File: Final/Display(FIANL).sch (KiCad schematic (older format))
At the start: 25 parts, among them U31 PAL16L8, U32 PAL16L8, U33 74LS374, U34 74LS374, U35 74LS374, U36 MAN71A, U37 MAN71A

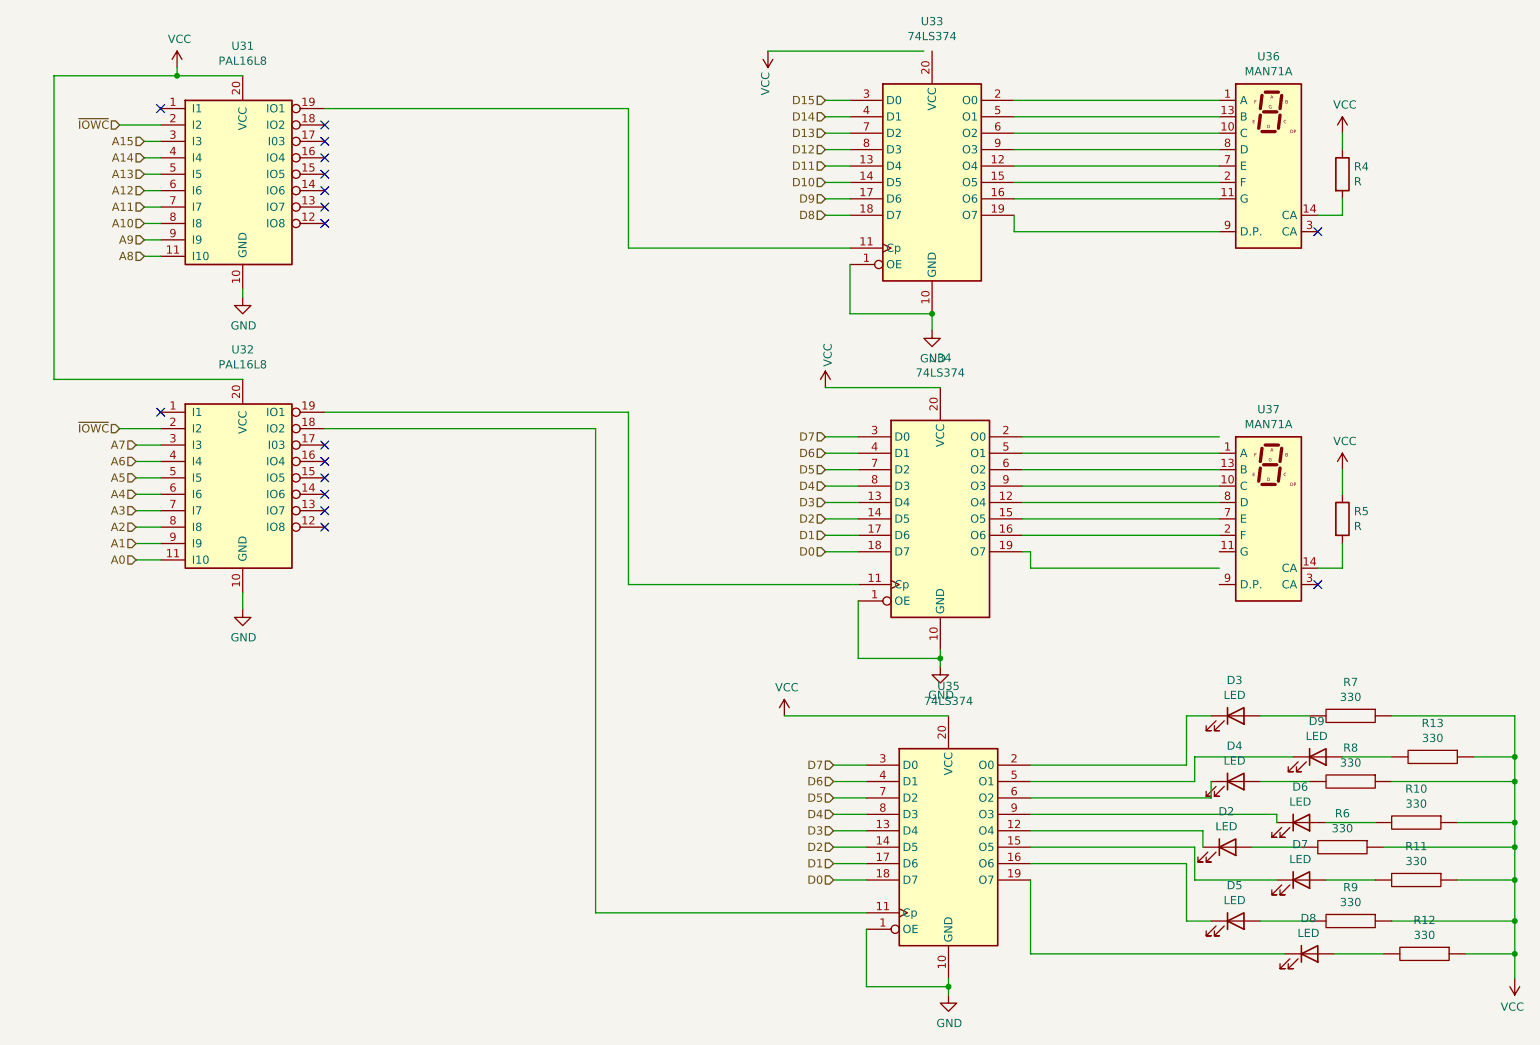
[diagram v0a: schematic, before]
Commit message: Final?
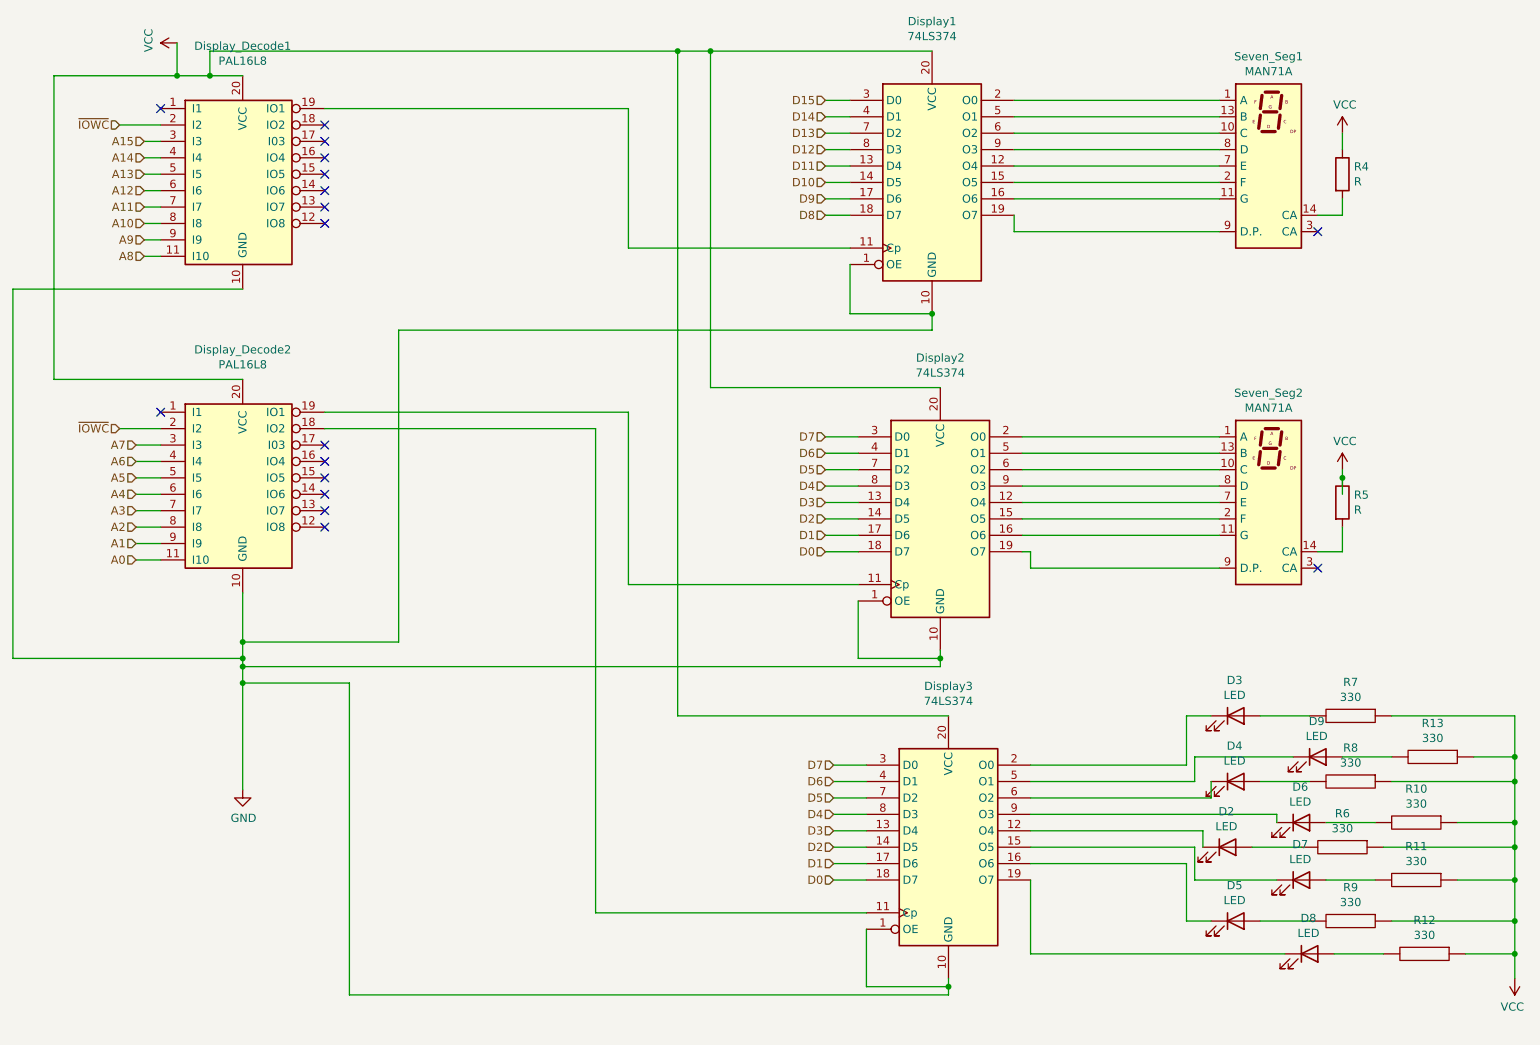
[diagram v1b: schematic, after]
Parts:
- renumbered U33 to Display1, U34 to Display2, U35 to Display3, U31 to Display_Decode1, U32 to Display_Decode2, U36 to Seven_Seg1, U37 to Seven_Seg2
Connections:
- net VCC: now also Display1.20 (VCC)
- net at Display2.12 (O4): now also Seven_Seg2.7 (E); no longer Seven_Seg2.8 (D)
- net at Display2.15 (O5): now also Seven_Seg2.2 (F); no longer Seven_Seg2.7 (E)
- net at Display2.16 (O6): now also Seven_Seg2.11 (G); no longer Seven_Seg2.2 (F)
- net at Display2.19 (O7): now also Seven_Seg2.9 (D.P.)
- net at Display2.2 (O0): now also Seven_Seg2.1 (A)
- net at Display2.5 (O1): now also Seven_Seg2.13 (B); no longer Seven_Seg2.1 (A)
- net at Display2.6 (O2): now also Seven_Seg2.10 (C); no longer Seven_Seg2.13 (B)
- net at Display2.9 (O3): now also Seven_Seg2.8 (D); no longer Seven_Seg2.10 (C)
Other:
- moved on the sheet: R5, Seven_Seg2
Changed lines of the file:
@@
 $Descr A4 11693 8268
 encoding utf-8
-Sheet 11 16
+Sheet 13 16
 Title ""
 Date ""
@@
 $EndDescr
 $Comp
-L 74xx:74LS374 U33
+L 74xx:74LS374 Display1
 U 1 1 607791B4
 P 7500 1450
-F 0 "U33" H 7500 2431 50  0000 C CNN
+F 0 "Display1" H 7500 2431 50  0000 C CNN
 F 1 "74LS374" H 7500 2340 50  0000 C CNN
 F 2 "" H 7500 1450 50  0001 C CNN
@@
 $EndComp
 $Comp
-L 74xx:74LS374 U34
+L 74xx:74LS374 Display2
 U 1 1 60775947
 P 7550 3500
-F 0 "U34" H 7550 4481 50  0000 C CNN
+F 0 "Display2" H 7550 4481 50  0000 C CNN
 F 1 "74LS374" H 7550 4390 50  0000 C CNN
 F 2 "" H 7550 3500 50  0001 C CNN
@@
 $EndComp
 $Comp
-L 74xx:74LS374 U35
+L 74xx:74LS374 Display3
 U 1 1 60778C07
 P 7600 5500
-F 0 "U35" H 7600 6481 50  0000 C CNN
+F 0 "Display3" H 7600 6481 50  0000 C CNN
 F 1 "74LS374" H 7600 6390 50  0000 C CNN
 F 2 "" H 7600 5500 50  0001 C CNN
@@
 Wire Wire Line
 	7100 5100 6900 5100
-$Comp
-L power:VCC #PWR057
-U 1 1 6079D8CA
-P 6850 2700
-F 0 "#PWR057" H 6850 2550 50  0001 C CNN
-F 1 "VCC" V 6865 2827 50  0000 L CNN
-F 2 "" H 6850 2700 50  0001 C CNN
-F 3 "" H 6850 2700 50  0001 C CNN
-	1    6850 2700
-	1    0    0    -1
-$EndComp
-$Comp
-L power:GND #PWR058
-U 1 1 607A1D53
-P 7600 6400
-F 0 "#PWR058" H 7600 6150 50  0001 C CNN
-F 1 "GND" H 7605 6227 50  0000 C CNN
-F 2 "" H 7600 6400 50  0001 C CNN
-F 3 "" H 7600 6400 50  0001 C CNN
-	1    7600 6400
-	1    0    0    -1
-$EndComp
 Wire Wire Line
 	7000 1950 7000 2250
@@
 	7050 4350 7550 4350
 $Comp
-L Display_Character:MAN71A U36
+L Display_Character:MAN71A Seven_Seg1
 U 1 1 6078B9DF
 P 9550 1350
-F 0 "U36" H 9550 2017 50  0000 C CNN
+F 0 "Seven_Seg1" H 9550 2017 50  0000 C CNN
 F 1 "MAN71A" H 9550 1926 50  0000 C CNN
 F 2 "Display_7Segment:MAN71A" H 9050 650 50  0001 L CNN
@@
 $EndComp
 $Comp
-L Display_Character:MAN71A U37
+L Display_Character:MAN71A Seven_Seg2
 U 1 1 6079109D
-P 9550 3500
-F 0 "U37" H 9550 4167 50  0000 C CNN
-F 1 "MAN71A" H 9550 4076 50  0000 C CNN
-F 2 "Display_7Segment:MAN71A" H 9050 2800 50  0001 L CNN
-F 3 "https://www.digchip.com/datasheets/parts/datasheet/161/MAN3640A-pdf.php" H 9560 3840 50  0001 L CNN
-	1    9550 3500
+P 9550 3400
+F 0 "Seven_Seg2" H 9550 4067 50  0000 C CNN
+F 1 "MAN71A" H 9550 3976 50  0000 C CNN
+F 2 "Display_7Segment:MAN71A" H 9050 2700 50  0001 L CNN
+F 3 "https://www.digchip.com/datasheets/parts/datasheet/161/MAN3640A-pdf.php" H 9560 3740 50  0001 L CNN
+	1    9550 3400
 	1    0    0    -1
 $EndComp
@@
 	5650 1850 7000 1850
 Wire Wire Line
-	3300 800  2900 800
-Wire Wire Line
-	2900 800  2900 750
+	3300 800  3100 800
 $Comp
 L power:VCC #PWR054
 U 1 1 607ECC89
-P 2900 750
-F 0 "#PWR054" H 2900 600 50  0001 C CNN
-F 1 "VCC" H 2915 923 50  0000 C CNN
-F 2 "" H 2900 750 50  0001 C CNN
-F 3 "" H 2900 750 50  0001 C CNN
-	1    2900 750
-	1    0    0    -1
-$EndComp
-$Comp
-L power:GND #PWR055
-U 1 1 607EDAEB
-P 3300 2150
-F 0 "#PWR055" H 3300 1900 50  0001 C CNN
-F 1 "GND" H 3305 1977 50  0000 C CNN
-F 2 "" H 3300 2150 50  0001 C CNN
-F 3 "" H 3300 2150 50  0001 C CNN
-	1    3300 2150
-	1    0    0    -1
+P 2900 600
+F 0 "#PWR054" H 2900 450 50  0001 C CNN
+F 1 "VCC" H 2915 773 50  0000 C CNN
+F 2 "" H 2900 600 50  0001 C CNN
+F 3 "" H 2900 600 50  0001 C CNN
+	1    2900 600
+	0    -1   -1   0
 $EndComp
 Wire Wire Line
 	2800 1100 2550 1100
 $Comp
-L Logic_Programmable:PAL16L8 U32
+L Logic_Programmable:PAL16L8 Display_Decode2
 U 1 1 607F2271
 P 3300 3350
-F 0 "U32" H 3300 4231 50  0000 C CNN
+F 0 "Display_Decode2" H 3300 4231 50  0000 C CNN
 F 1 "PAL16L8" H 3300 4140 50  0000 C CNN
 F 2 "" H 3300 3350 50  0001 C CNN
@@
 	2150 800  2900 800
 Connection ~ 2900 800
-Wire Wire Line
-	3300 2100 3300 2150
-Wire Wire Line
-	3300 3950 3300 4050
 $Comp
 L power:GND #PWR056
 U 1 1 607FE1E1
-P 3300 4050
-F 0 "#PWR056" H 3300 3800 50  0001 C CNN
-F 1 "GND" H 3305 3877 50  0000 C CNN
-F 2 "" H 3300 4050 50  0001 C CNN
-F 3 "" H 3300 4050 50  0001 C CNN
-	1    3300 4050
+P 3300 5150
+F 0 "#PWR056" H 3300 4900 50  0001 C CNN
+F 1 "GND" H 3305 4977 50  0000 C CNN
+F 2 "" H 3300 5150 50  0001 C CNN
+F 3 "" H 3300 5150 50  0001 C CNN
+	1    3300 5150
 	1    0    0    -1
 $EndComp
@@
 	2800 2950 2550 2950
 $Comp
-L Logic_Programmable:PAL16L8 U31
+L Logic_Programmable:PAL16L8 Display_Decode1
 U 1 1 607E2663
 P 3300 1500
-F 0 "U31" H 3300 2381 50  0000 C CNN
+F 0 "Display_Decode1" H 3300 2381 50  0000 C CNN
 F 1 "PAL16L8" H 3300 2290 50  0000 C CNN
 F 2 "" H 3300 1500 50  0001 C CNN
@@
 	10000 1650 10000 1550
 Wire Wire Line
-	9850 3800 10000 3800
-Wire Wire Line
-	10000 3800 10000 3650
+	9850 3700 10000 3700
+Wire Wire Line
+	10000 3700 10000 3550
 $Comp
 L Device:R R4
@@
 L Device:R R5
 U 1 1 607D65C2
-P 10000 3500
-F 0 "R5" H 10070 3546 50  0000 L CNN
-F 1 "R" H 10070 3455 50  0000 L CNN
-F 2 "" V 9930 3500 50  0001 C CNN
-F 3 "~" H 10000 3500 50  0001 C CNN
-	1    10000 3500
+P 10000 3400
+F 0 "R5" H 10070 3446 50  0000 L CNN
+F 1 "R" H 10070 3355 50  0000 L CNN
+F 2 "" V 9930 3400 50  0001 C CNN
+F 3 "~" H 10000 3400 50  0001 C CNN
+	1    10000 3400
 	1    0    0    -1
 $EndComp
@@
 	10000 1250 10000 1150
 Wire Wire Line
-	10000 3350 10000 3200
+	10000 3350 10000 3250
 $Comp
 L power:VCC #PWR059
@@
 NoConn ~ 3800 3550
 NoConn ~ 9850 1750
-NoConn ~ 9850 3900
 Wire Wire Line
 	5450 2950 5450 5900
@@
 	7550 4350 7550 4300
 Connection ~ 7550 4350
-$Comp
-L power:GND #PWR0105
-U 1 1 60A72376
-P 7550 4400
-F 0 "#PWR0105" H 7550 4150 50  0001 C CNN
-F 1 "GND" H 7555 4227 50  0000 C CNN
-F 2 "" H 7550 4400 50  0001 C CNN
-F 3 "" H 7550 4400 50  0001 C CNN
-	1    7550 4400
-	1    0    0    -1
-$EndComp
-$Comp
-L power:GND #PWR0102
-U 1 1 60A729AF
-P 7500 2350
-F 0 "#PWR0102" H 7500 2100 50  0001 C CNN
-F 1 "GND" H 7505 2177 50  0000 C CNN
-F 2 "" H 7500 2350 50  0001 C CNN
-F 3 "" H 7500 2350 50  0001 C CNN
-	1    7500 2350
-	1    0    0    -1
-$EndComp
-Wire Wire Line
-	7450 650  6500 650
-Wire Wire Line
-	7550 2700 6850 2700
-Wire Wire Line
-	7600 4700 6600 4700
-$Comp
-L power:VCC #PWR0103
-U 1 1 60A94EE1
-P 6600 4700
-F 0 "#PWR0103" H 6600 4550 50  0001 C CNN
-F 1 "VCC" H 6615 4873 50  0000 C CNN
-F 2 "" H 6600 4700 50  0001 C CNN
-F 3 "" H 6600 4700 50  0001 C CNN
-	1    6600 4700
-	1    0    0    -1
-$EndComp
-$Comp
-L power:VCC #PWR0104
-U 1 1 60A9BDC3
-P 6500 650
-F 0 "#PWR0104" H 6500 500 50  0001 C CNN
-F 1 "VCC" V 6515 777 50  0000 L CNN
-F 2 "" H 6500 650 50  0001 C CNN
-F 3 "" H 6500 650 50  0001 C CNN
-	1    6500 650
-	-1   0    0    1
-$EndComp
+Wire Wire Line
+	3300 3950 3300 4250
+Wire Wire Line
+	3300 2100 1900 2100
+Wire Wire Line
+	1900 2100 1900 4350
+Wire Wire Line
+	1900 4350 3300 4350
+Connection ~ 3300 4350
+Wire Wire Line
+	3300 4350 3300 4400
+Wire Wire Line
+	2900 600  2900 800
+Wire Wire Line
+	3100 650  3100 800
+Connection ~ 3100 800
+Wire Wire Line
+	3100 800  2900 800
+Wire Wire Line
+	3100 650  5950 650
+Wire Wire Line
+	7600 6400 3950 6400
+Wire Wire Line
+	3950 6400 3950 4500
+Wire Wire Line
+	3950 4500 3300 4500
+Connection ~ 3300 4500
+Wire Wire Line
+	7550 4400 3300 4400
+Connection ~ 3300 4400
+Wire Wire Line
+	3300 4400 3300 4500
+Wire Wire Line
+	7500 2350 4250 2350
+Wire Wire Line
+	4250 2350 4250 4250
+Wire Wire Line
+	4250 4250 3300 4250
+Connection ~ 3300 4250
+Wire Wire Line
+	3300 4250 3300 4350
+Wire Wire Line
+	3300 4500 3300 5150
+Wire Wire Line
+	6150 2700 6150 650
+Wire Wire Line
+	6150 2700 7550 2700
+Connection ~ 6150 650
+Wire Wire Line
+	6150 650  7500 650
+Wire Wire Line
+	5950 4700 5950 650
+Wire Wire Line
+	5950 4700 7600 4700
+Connection ~ 5950 650
+Wire Wire Line
+	5950 650  6150 650
+Connection ~ 10000 3250
+Wire Wire Line
+	10000 3250 10000 3200
+NoConn ~ 9850 3800
 $EndSCHEMATC

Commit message: Hopefully the board is here
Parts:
- D2, D3, D4, D5, D6, D7, D8, D9: footprint (none) -> LED_THT:LED_D1.8mm_W1.8mm_H2.4mm_Horizontal_O1.27mm_Z4.9mm
- Display1, Display2, Display3, Display_Decode1, Display_Decode2: footprint (none) -> Package_DIP:DIP-20_W7.62mm
- R10, R11, R12, R13, R4, R5, R6, R7, R8, R9: footprint (none) -> Resistor_THT:R_Axial_DIN0204_L3.6mm_D1.6mm_P2.54mm_Vertical
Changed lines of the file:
@@
 F 0 "Display1" H 7500 2431 50  0000 C CNN
 F 1 "74LS374" H 7500 2340 50  0000 C CNN
-F 2 "" H 7500 1450 50  0001 C CNN
+F 2 "Package_DIP:DIP-20_W7.62mm" H 7500 1450 50  0001 C CNN
 F 3 "http://www.ti.com/lit/gpn/sn74LS374" H 7500 1450 50  0001 C CNN
 	1    7500 1450
@@
 F 0 "Display2" H 7550 4481 50  0000 C CNN
 F 1 "74LS374" H 7550 4390 50  0000 C CNN
-F 2 "" H 7550 3500 50  0001 C CNN
+F 2 "Package_DIP:DIP-20_W7.62mm" H 7550 3500 50  0001 C CNN
 F 3 "http://www.ti.com/lit/gpn/sn74LS374" H 7550 3500 50  0001 C CNN
 	1    7550 3500
@@
 F 0 "Display3" H 7600 6481 50  0000 C CNN
 F 1 "74LS374" H 7600 6390 50  0000 C CNN
-F 2 "" H 7600 5500 50  0001 C CNN
+F 2 "Package_DIP:DIP-20_W7.62mm" H 7600 5500 50  0001 C CNN
 F 3 "http://www.ti.com/lit/gpn/sn74LS374" H 7600 5500 50  0001 C CNN
 	1    7600 5500
@@
 F 0 "Display_Decode2" H 3300 4231 50  0000 C CNN
 F 1 "PAL16L8" H 3300 4140 50  0000 C CNN
-F 2 "" H 3300 3350 50  0001 C CNN
+F 2 "Package_DIP:DIP-20_W7.62mm" H 3300 3350 50  0001 C CNN
 F 3 "" H 3300 3350 50  0001 C CNN
 	1    3300 3350
@@
 F 0 "Display_Decode1" H 3300 2381 50  0000 C CNN
 F 1 "PAL16L8" H 3300 2290 50  0000 C CNN
-F 2 "" H 3300 1500 50  0001 C CNN
+F 2 "Package_DIP:DIP-20_W7.62mm" H 3300 1500 50  0001 C CNN
 F 3 "" H 3300 1500 50  0001 C CNN
 	1    3300 1500
@@
 F 0 "R7" V 9845 4700 50  0000 C CNN
 F 1 "330" V 9936 4700 50  0000 C CNN
-F 2 "" H 10050 4700 50  0001 C CNN
+F 2 "Resistor_THT:R_Axial_DIN0204_L3.6mm_D1.6mm_P2.54mm_Vertical" H 10050 4700 50  0001 C CNN
 F 3 "~" H 10050 4700 50  0001 C CNN
 	1    10050 4700
@@
 F 0 "R13" V 10345 4950 50  0000 C CNN
 F 1 "330" V 10436 4950 50  0000 C CNN
-F 2 "" H 10550 4950 50  0001 C CNN
+F 2 "Resistor_THT:R_Axial_DIN0204_L3.6mm_D1.6mm_P2.54mm_Vertical" H 10550 4950 50  0001 C CNN
 F 3 "~" H 10550 4950 50  0001 C CNN
 	1    10550 4950
@@
 F 0 "R8" V 9845 5100 50  0000 C CNN
 F 1 "330" V 9936 5100 50  0000 C CNN
-F 2 "" H 10050 5100 50  0001 C CNN
+F 2 "Resistor_THT:R_Axial_DIN0204_L3.6mm_D1.6mm_P2.54mm_Vertical" H 10050 5100 50  0001 C CNN
 F 3 "~" H 10050 5100 50  0001 C CNN
 	1    10050 5100
@@
 F 0 "R10" V 10245 5350 50  0000 C CNN
 F 1 "330" V 10336 5350 50  0000 C CNN
-F 2 "" H 10450 5350 50  0001 C CNN
+F 2 "Resistor_THT:R_Axial_DIN0204_L3.6mm_D1.6mm_P2.54mm_Vertical" H 10450 5350 50  0001 C CNN
 F 3 "~" H 10450 5350 50  0001 C CNN
 	1    10450 5350
@@
 F 0 "R11" V 10245 5700 50  0000 C CNN
 F 1 "330" V 10336 5700 50  0000 C CNN
-F 2 "" H 10450 5700 50  0001 C CNN
+F 2 "Resistor_THT:R_Axial_DIN0204_L3.6mm_D1.6mm_P2.54mm_Vertical" H 10450 5700 50  0001 C CNN
 F 3 "~" H 10450 5700 50  0001 C CNN
 	1    10450 5700
@@
 F 0 "R6" V 9795 5500 50  0000 C CNN
 F 1 "330" V 9886 5500 50  0000 C CNN
-F 2 "" H 10000 5500 50  0001 C CNN
+F 2 "Resistor_THT:R_Axial_DIN0204_L3.6mm_D1.6mm_P2.54mm_Vertical" H 10000 5500 50  0001 C CNN
 F 3 "~" H 10000 5500 50  0001 C CNN
 	1    10000 5500
@@
 F 0 "R9" V 9845 5950 50  0000 C CNN
 F 1 "330" V 9936 5950 50  0000 C CNN
-F 2 "" H 10050 5950 50  0001 C CNN
+F 2 "Resistor_THT:R_Axial_DIN0204_L3.6mm_D1.6mm_P2.54mm_Vertical" H 10050 5950 50  0001 C CNN
 F 3 "~" H 10050 5950 50  0001 C CNN
 	1    10050 5950
@@
 F 0 "R12" V 10295 6150 50  0000 C CNN
 F 1 "330" V 10386 6150 50  0000 C CNN
-F 2 "" H 10500 6150 50  0001 C CNN
+F 2 "Resistor_THT:R_Axial_DIN0204_L3.6mm_D1.6mm_P2.54mm_Vertical" H 10500 6150 50  0001 C CNN
 F 3 "~" H 10500 6150 50  0001 C CNN
 	1    10500 6150
@@
 F 0 "D3" H 9343 4917 50  0000 C CNN
 F 1 "LED" H 9343 4826 50  0000 C CNN
-F 2 "" H 9350 4700 50  0001 C CNN
+F 2 "LED_THT:LED_D1.8mm_W1.8mm_H2.4mm_Horizontal_O1.27mm_Z4.9mm" H 9350 4700 50  0001 C CNN
 F 3 "~" H 9350 4700 50  0001 C CNN
 	1    9350 4700
@@
 F 0 "D5" H 9343 6167 50  0000 C CNN
 F 1 "LED" H 9343 6076 50  0000 C CNN
-F 2 "" H 9350 5950 50  0001 C CNN
+F 2 "LED_THT:LED_D1.8mm_W1.8mm_H2.4mm_Horizontal_O1.27mm_Z4.9mm" H 9350 5950 50  0001 C CNN
 F 3 "~" H 9350 5950 50  0001 C CNN
 	1    9350 5950
@@
 F 0 "D4" H 9343 5317 50  0000 C CNN
 F 1 "LED" H 9343 5226 50  0000 C CNN
-F 2 "" H 9350 5100 50  0001 C CNN
+F 2 "LED_THT:LED_D1.8mm_W1.8mm_H2.4mm_Horizontal_O1.27mm_Z4.9mm" H 9350 5100 50  0001 C CNN
 F 3 "~" H 9350 5100 50  0001 C CNN
 	1    9350 5100
@@
 F 0 "D8" H 9793 6367 50  0000 C CNN
 F 1 "LED" H 9793 6276 50  0000 C CNN
-F 2 "" H 9800 6150 50  0001 C CNN
+F 2 "LED_THT:LED_D1.8mm_W1.8mm_H2.4mm_Horizontal_O1.27mm_Z4.9mm" H 9800 6150 50  0001 C CNN
 F 3 "~" H 9800 6150 50  0001 C CNN
 	1    9800 6150
@@
 F 0 "D9" H 9843 5167 50  0000 C CNN
 F 1 "LED" H 9843 5076 50  0000 C CNN
-F 2 "" H 9850 4950 50  0001 C CNN
+F 2 "LED_THT:LED_D1.8mm_W1.8mm_H2.4mm_Horizontal_O1.27mm_Z4.9mm" H 9850 4950 50  0001 C CNN
 F 3 "~" H 9850 4950 50  0001 C CNN
 	1    9850 4950
@@
 F 0 "D7" H 9743 5917 50  0000 C CNN
 F 1 "LED" H 9743 5826 50  0000 C CNN
-F 2 "" H 9750 5700 50  0001 C CNN
+F 2 "LED_THT:LED_D1.8mm_W1.8mm_H2.4mm_Horizontal_O1.27mm_Z4.9mm" H 9750 5700 50  0001 C CNN
 F 3 "~" H 9750 5700 50  0001 C CNN
 	1    9750 5700
@@
 F 0 "D2" H 9293 5717 50  0000 C CNN
 F 1 "LED" H 9293 5626 50  0000 C CNN
-F 2 "" H 9300 5500 50  0001 C CNN
+F 2 "LED_THT:LED_D1.8mm_W1.8mm_H2.4mm_Horizontal_O1.27mm_Z4.9mm" H 9300 5500 50  0001 C CNN
 F 3 "~" H 9300 5500 50  0001 C CNN
 	1    9300 5500
@@
 F 0 "D6" H 9743 5567 50  0000 C CNN
 F 1 "LED" H 9743 5476 50  0000 C CNN
-F 2 "" H 9750 5350 50  0001 C CNN
+F 2 "LED_THT:LED_D1.8mm_W1.8mm_H2.4mm_Horizontal_O1.27mm_Z4.9mm" H 9750 5350 50  0001 C CNN
 F 3 "~" H 9750 5350 50  0001 C CNN
 	1    9750 5350
@@
 F 0 "R4" H 10070 1446 50  0000 L CNN
 F 1 "R" H 10070 1355 50  0000 L CNN
-F 2 "" V 9930 1400 50  0001 C CNN
+F 2 "Resistor_THT:R_Axial_DIN0204_L3.6mm_D1.6mm_P2.54mm_Vertical" V 9930 1400 50  0001 C CNN
 F 3 "~" H 10000 1400 50  0001 C CNN
 	1    10000 1400
@@
 F 0 "R5" H 10070 3446 50  0000 L CNN
 F 1 "R" H 10070 3355 50  0000 L CNN
-F 2 "" V 9930 3400 50  0001 C CNN
+F 2 "Resistor_THT:R_Axial_DIN0204_L3.6mm_D1.6mm_P2.54mm_Vertical" V 9930 3400 50  0001 C CNN
 F 3 "~" H 10000 3400 50  0001 C CNN
 	1    10000 3400
